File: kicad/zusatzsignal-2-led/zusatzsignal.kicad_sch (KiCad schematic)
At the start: 2 parts

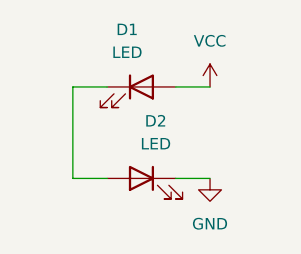
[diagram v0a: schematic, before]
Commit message: MSv2
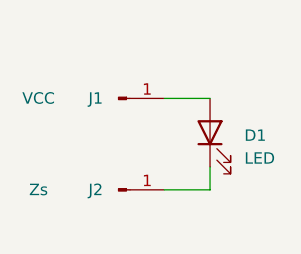
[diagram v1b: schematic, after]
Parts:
- removed D2: LED, LED_SMD:LED_0603_1608Metric, symbol Device:LED
- added J1: VCC, Connector_Wire:SolderWirePad_1x01_SMD_1x2mm, symbol Connector:Conn_01x01_Male
- added J2: Zs, Connector_Wire:SolderWirePad_1x01_SMD_1x2mm, symbol Connector:Conn_01x01_Male
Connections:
- net at D1.1 (K): now also J2.1 (Pin_1)
- net VCC: no longer names the net of D1.2 (A)
- net VCC: now also J1.1 (Pin_1)
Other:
- moved on the sheet: D1
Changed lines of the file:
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@@
 (kicad_sch (version 20211123) (generator eeschema)
   (paper "A4")
-  (wire (pts (xy 74.93 64.77) (xy 71.12 64.77))
+  (wire (pts (xy 81.28 76.2) (xy 86.36 76.2))
     (stroke (width 0) (type default) (color 0 0 0 0))
   )
-  (wire (pts (xy 71.12 74.93) (xy 74.93 74.93))
+  (wire (pts (xy 86.36 76.2) (xy 86.36 73.66))
     (stroke (width 0) (type default) (color 0 0 0 0))
   )
-  (wire (pts (xy 82.55 74.93) (xy 86.36 74.93))
+  (wire (pts (xy 81.28 66.04) (xy 86.36 66.04))
     (stroke (width 0) (type default) (color 0 0 0 0))
   )
-  (wire (pts (xy 71.12 64.77) (xy 71.12 74.93))
-    (stroke (width 0) (type default) (color 0 0 0 0))
-  )
-  (wire (pts (xy 82.55 64.77) (xy 86.36 64.77))
-    (stroke (width 0) (type default) (color 0 0 0 0))
-  )
-  (symbol (lib_id "Device:LED") (at 78.74 74.93 0) (mirror y) (unit 1)
+  (symbol (lib_id "Device:LED") (at 86.36 69.85 90) (unit 1)
     (in_bom yes) (on_board yes) (fields_autoplaced)
-    (property "Reference" "D2" (id 0) (at 80.3275 68.58 0))
-    (property "Value" "LED" (id 1) (at 80.3275 71.12 0))
-    (property "Footprint" "LED_SMD:LED_0603_1608Metric" (id 2) (at 78.74 74.93 0)
+    (property "Reference" "D1" (id 0) (at 90.17 70.1674 90)
+      (effects (font (size 1.27 1.27)) (justify right))
+    )
+    (property "Value" "LED" (id 1) (at 90.17 72.7074 90)
+      (effects (font (size 1.27 1.27)) (justify right))
+    )
+    (property "Footprint" "LED_SMD:LED_0603_1608Metric" (id 2) (at 86.36 69.85 0)
       (effects (font (size 1.27 1.27)) hide)
     )
-    (property "Datasheet" "~" (id 3) (at 78.74 74.93 0)
+    (property "Datasheet" "~" (id 3) (at 86.36 69.85 0)
       (effects (font (size 1.27 1.27)) hide)
     )
@@
     (pin "2")
   )
-  (symbol (lib_id "power:VCC") (at 86.36 64.77 0) (unit 1)
-    (in_bom yes) (on_board yes) (fields_autoplaced)
-    (property "Reference" "#PWR?" (id 0) (at 86.36 68.58 0)
+  (symbol (lib_id "Connector:Conn_01x01_Male") (at 76.2 76.2 0) (unit 1)
+    (in_bom yes) (on_board yes)
+    (property "Reference" "J2" (id 0) (at 73.66 76.2 0))
+    (property "Value" "Zs" (id 1) (at 67.31 76.2 0))
+    (property "Footprint" "Connector_Wire:SolderWirePad_1x01_SMD_1x2mm" (id 2) (at 76.2 76.2 0)
       (effects (font (size 1.27 1.27)) hide)
     )
-    (property "Value" "VCC" (id 1) (at 86.36 59.69 0))
-    (property "Footprint" "Connector_Wire:SolderWirePad_1x01_SMD_1x2mm" (id 2) (at 86.36 64.77 0)
-      (effects (font (size 1.27 1.27)) hide)
-    )
-    (property "Datasheet" "" (id 3) (at 86.36 64.77 0)
+    (property "Datasheet" "~" (id 3) (at 76.2 76.2 0)
       (effects (font (size 1.27 1.27)) hide)
     )
     (pin "1")
   )
-  (symbol (lib_id "power:GND") (at 86.36 74.93 0) (unit 1)
-    (in_bom yes) (on_board yes) (fields_autoplaced)
-    (property "Reference" "#PWR?" (id 0) (at 86.36 81.28 0)
+  (symbol (lib_id "Connector:Conn_01x01_Male") (at 76.2 66.04 0) (unit 1)
+    (in_bom yes) (on_board yes)
+    (property "Reference" "J1" (id 0) (at 73.66 66.04 0))
+    (property "Value" "VCC" (id 1) (at 67.31 66.04 0))
+    (property "Footprint" "Connector_Wire:SolderWirePad_1x01_SMD_1x2mm" (id 2) (at 76.2 66.04 0)
       (effects (font (size 1.27 1.27)) hide)
     )
-    (property "Value" "GND" (id 1) (at 86.36 80.01 0))
-    (property "Footprint" "Connector_Wire:SolderWirePad_1x01_SMD_1x2mm" (id 2) (at 86.36 74.93 0)
-      (effects (font (size 1.27 1.27)) hide)
-    )
-    (property "Datasheet" "" (id 3) (at 86.36 74.93 0)
+    (property "Datasheet" "~" (id 3) (at 76.2 66.04 0)
       (effects (font (size 1.27 1.27)) hide)
     )
     (pin "1")
-  )
-  (symbol (lib_id "Device:LED") (at 78.74 64.77 0) (unit 1)
-    (in_bom yes) (on_board yes) (fields_autoplaced)
-    (property "Reference" "D1" (id 0) (at 77.1525 58.42 0))
-    (property "Value" "LED" (id 1) (at 77.1525 60.96 0))
-    (property "Footprint" "LED_SMD:LED_0603_1608Metric" (id 2) (at 78.74 64.77 0)
-      (effects (font (size 1.27 1.27)) hide)
-    )
-    (property "Datasheet" "~" (id 3) (at 78.74 64.77 0)
-      (effects (font (size 1.27 1.27)) hide)
-    )
-    (pin "1")
-    (pin "2")
   )
   (sheet_instances
@@
   )
   (symbol_instances
-    (path "/64bc9de5-51b6-4885-a9f3-c002ef3bb482"
-      (reference "#PWR?") (unit 1) (value "VCC") (footprint "Connector_Wire:SolderWirePad_1x01_SMD_1x2mm")
-    )
-    (path "/9711282b-7f91-45c9-8f45-027328949a6b"
-      (reference "#PWR?") (unit 1) (value "GND") (footprint "Connector_Wire:SolderWirePad_1x01_SMD_1x2mm")
-    )
     (path "/a3f3a018-6a6b-4914-95d4-b6f25692820f"
       (reference "D1") (unit 1) (value "LED") (footprint "LED_SMD:LED_0603_1608Metric")
     )
-    (path "/51e081dd-14da-453b-ad0a-f912cce13100"
-      (reference "D2") (unit 1) (value "LED") (footprint "LED_SMD:LED_0603_1608Metric")
+    (path "/ebda1544-61d5-4166-a2e9-fde8904cbfc1"
+      (reference "J1") (unit 1) (value "VCC") (footprint "Connector_Wire:SolderWirePad_1x01_SMD_1x2mm")
+    )
+    (path "/e51e5768-e1af-448e-8d73-2a64bafc6c39"
+      (reference "J2") (unit 1) (value "Zs") (footprint "Connector_Wire:SolderWirePad_1x01_SMD_1x2mm")
     )
   )
